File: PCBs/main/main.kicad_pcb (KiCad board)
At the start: 2 copper layers, 2 parts, among them J4 Conn_02x10_Odd_Even

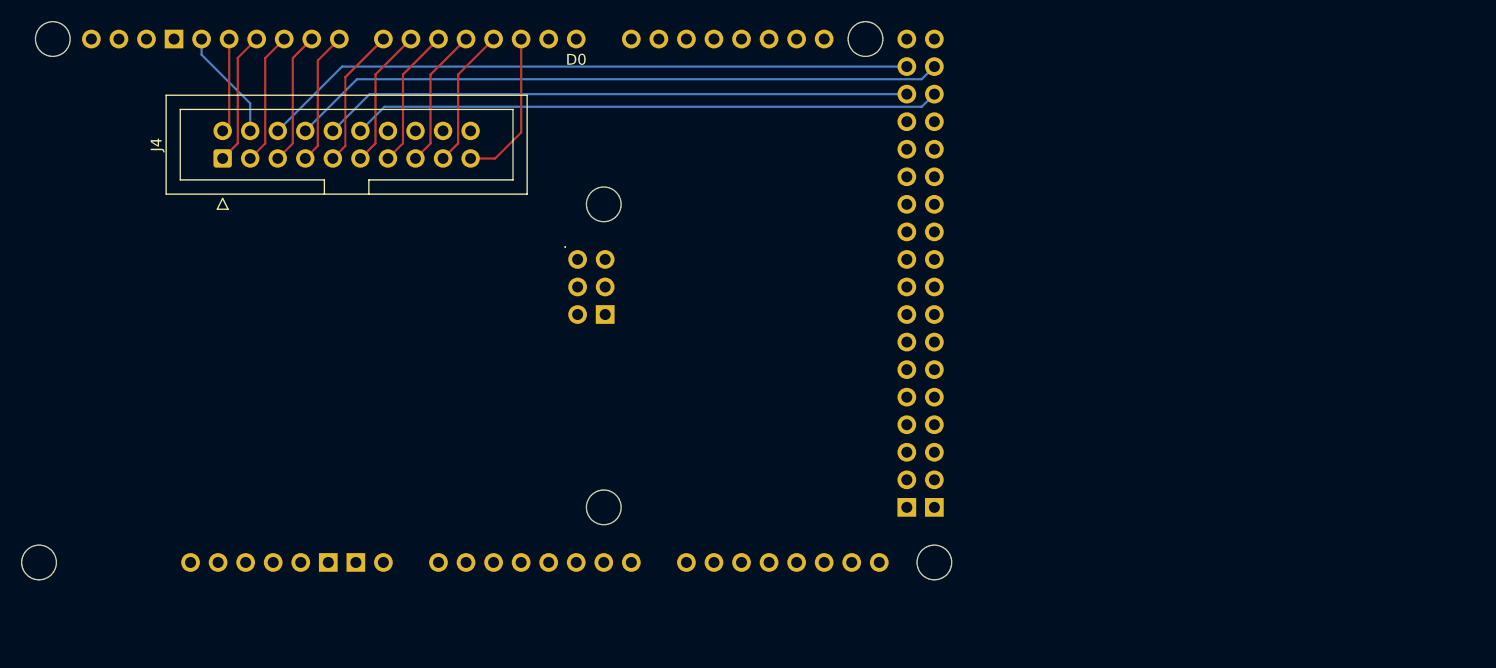
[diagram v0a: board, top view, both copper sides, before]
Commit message: work on first prototype for the boards
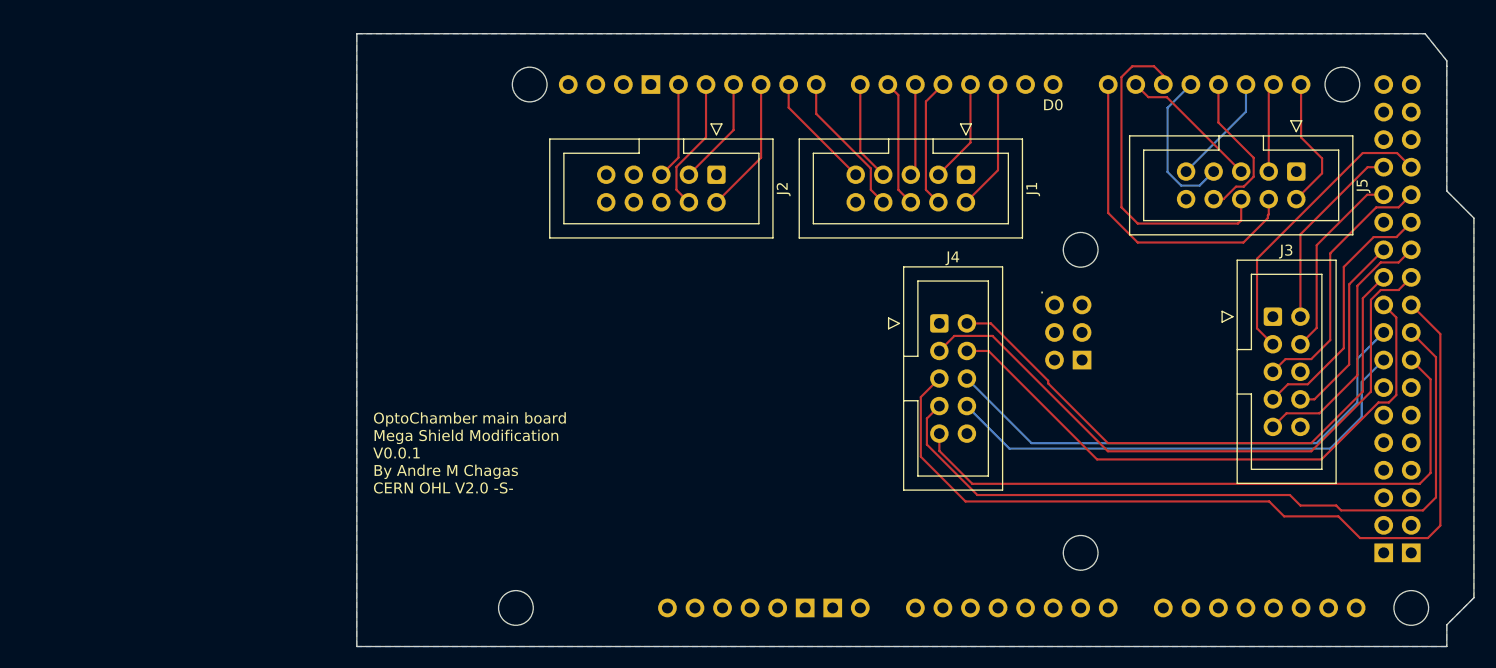
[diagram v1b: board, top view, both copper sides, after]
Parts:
- removed A1: Arduino_Mega2560_R3_Shield, PCM_arduino-library:Arduino_Mega2560_R3_Shield
- added A2: Arduino_Mega2560_R3_Shield, PCM_arduino-library:Arduino_Mega2560_R3_Shield, F.Cu at (87.2, 90.5)
- added J1: Conn_02x05_Counter_Clockwise, Connector_IDC:IDC-Header_2x05_P2.54mm_Vertical, F.Cu at (142.7, 48.0)
- added J2: Conn_02x05_Counter_Clockwise, Connector_IDC:IDC-Header_2x05_P2.54mm_Vertical, F.Cu at (119.7, 48.0)
- added J3: Conn_02x05_Counter_Clockwise, Connector_IDC:IDC-Header_2x05_P2.54mm_Vertical, F.Cu at (171.0, 61.1)
- added J5: chambers 9-10, Connector_IDC:IDC-Header_2x05_P2.54mm_Vertical, F.Cu at (173.1, 47.7)
- J4: value Conn_02x10_Odd_Even -> Conn_02x05_Counter_Clockwise; footprint Connector_IDC:IDC-Header_2x10_P2.54mm_Vertical -> Connector_IDC:IDC-Header_2x05_P2.54mm_Vertical
- moved J4 67.8 mm to (140.2, 61.7), turned to 0 degrees
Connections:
- J4 pad 1: Net-(J4-Pin_1) -> GND
- J4 pad 10: Net-(J4-Pin_10) -> GND
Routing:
- net Net-(J4-Pin_5): track 12.3 -> 80.9 mm
- net Net-(J4-Pin_7): track 12.3 -> 70.1 mm
- net Net-(J4-Pin_10): track 54.3 -> 0.00 mm
- net Net-(J4-Pin_12): track 54.3 -> 0.00 mm
- net Net-(J4-Pin_3): track 12.3 -> 60.1 mm
- net Net-(J4-Pin_9): track 12.9 -> 59.7 mm
- net Net-(J4-Pin_2): track 8.72 -> 54.5 mm
- net Net-(J4-Pin_4): track 10.3 -> 55.0 mm
- net Net-(A2-D16/TX2): track 0.00 -> 31.2 mm
- net Net-(A2-D14/TX3): track 0.00 -> 30.4 mm
- net Net-(J3-Pin_3): track 0.00 -> 27.3 mm
- net Net-(J3-Pin_9): track 0.00 -> 24.4 mm
- net Net-(J3-Pin_5): track 0.00 -> 24.2 mm
- net Net-(J3-Pin_7): track 0.00 -> 23.9 mm
- net Net-(J3-Pin_4): track 0.00 -> 17.9 mm
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- added copper zone on B.Cu, net GND
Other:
- board outline added: 103 x 56.5 mm
- board text added: "OptoChamber main board Mega Shield Modification V0.0.1 By Andre M Chagas CERN OHL V2.0 -S-"
